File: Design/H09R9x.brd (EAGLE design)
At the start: 34.6 x 30 mm, 24 parts, among them P1 HEXABIT_17.32, U1 STM32F091CBU6, U2 TSD305-1C55, X1 XTALL_CSTCE8M00G52

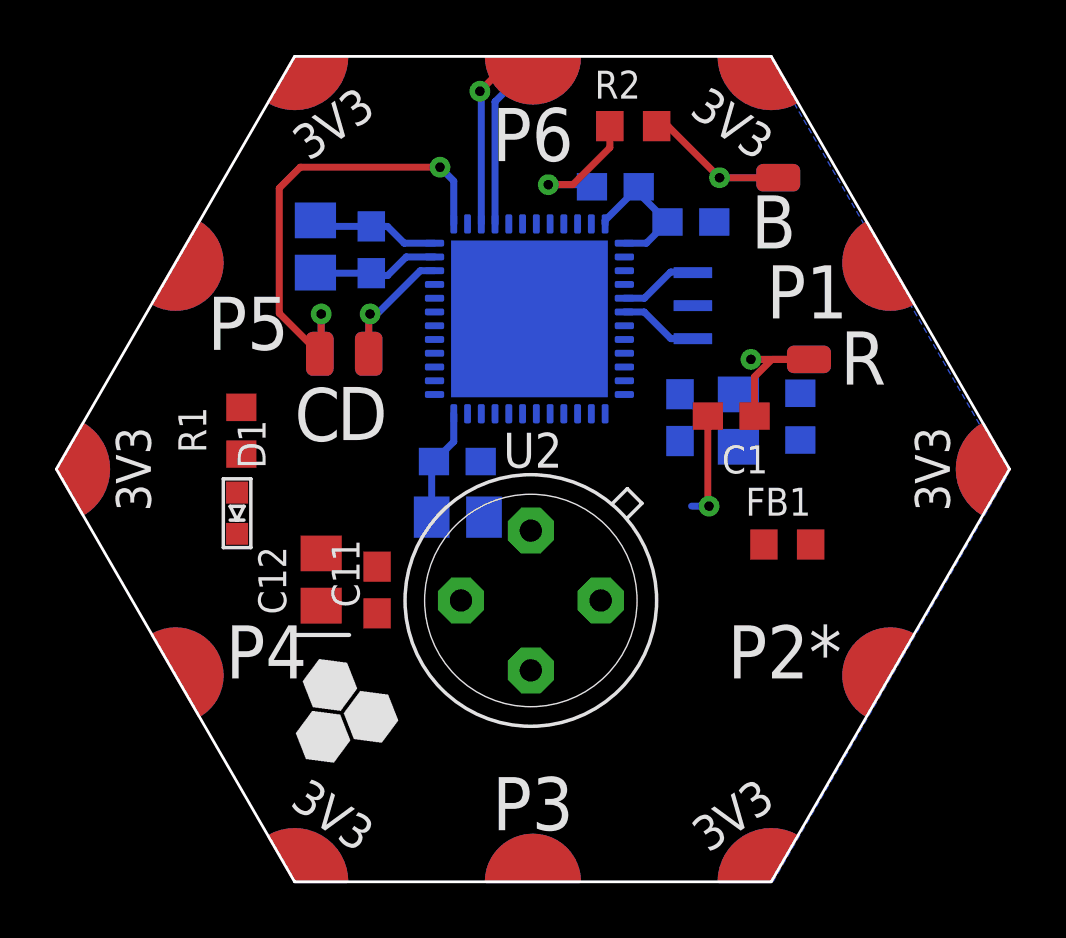
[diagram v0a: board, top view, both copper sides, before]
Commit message: brd edit
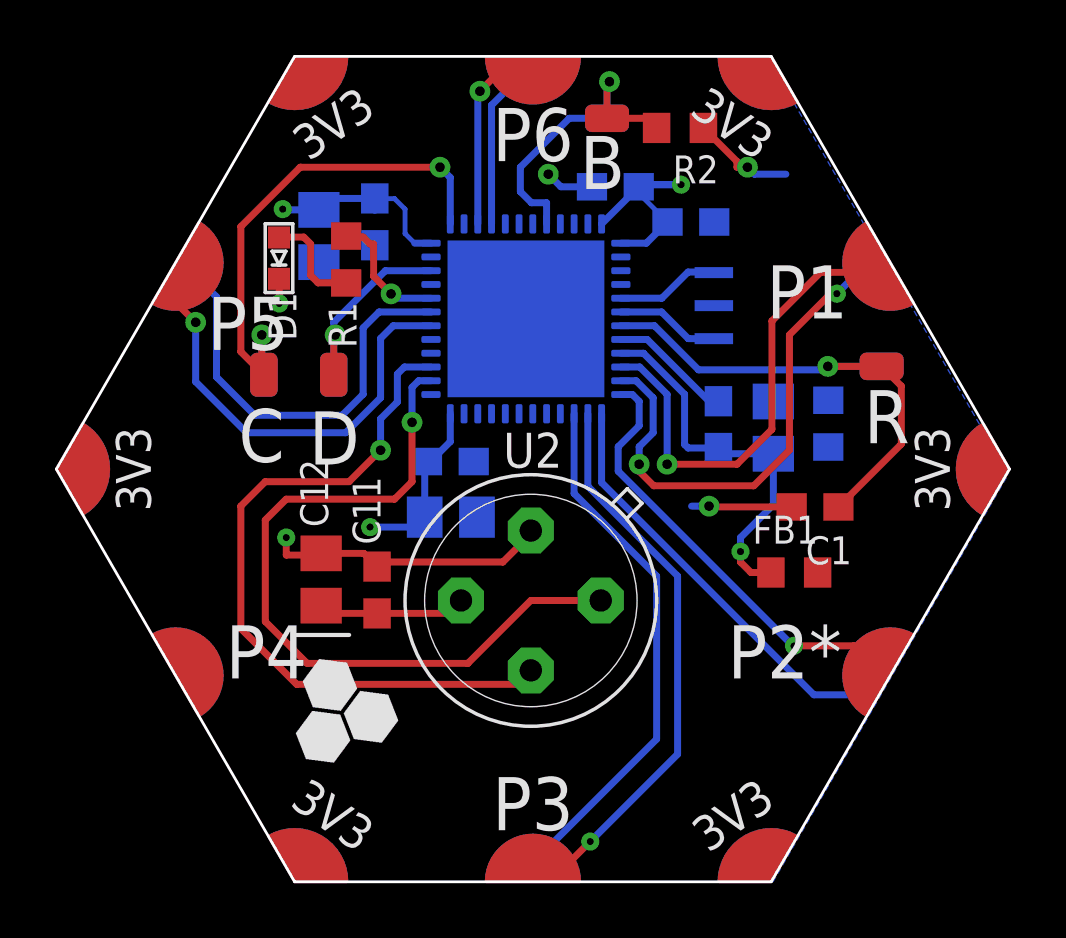
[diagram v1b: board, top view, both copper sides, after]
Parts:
- moved D1 9.40 mm to (25.4, 42.3)
- moved R1 7.30 mm to (27.8, 42.2)
- moved B 6.59 mm to (37.3, 47.4)
- moved C1 4.49 mm to (44.9, 33.2)
- moved R 2.65 mm to (47.3, 38.4), turned to 180 degrees
- moved C 2.17 mm to (24.8, 38.0)
- moved R2 1.70 mm to (40.0, 47.0), turned to 180 degrees
- moved D 1.48 mm to (27.4, 38.0)
- moved C5 1.42 mm to (41.4, 36.2)
- moved C2 1.30 mm to (43.4, 36.1)
- moved FB1 1.05 mm to (44.1, 30.9)
- moved R3 1.05 mm to (45.4, 36.3)
- moved C7 1.02 mm to (28.9, 43.6)
- moved X1 0.76 mm to (41.2, 40.6)
- moved C4 0.40 mm to (26.8, 43.1)
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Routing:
- net I2C2_SCL: track 0.00 -> 27.6 mm, vias 0 -> 1
- net I2C2_SDA: track 0.00 -> 26.3 mm, vias 0 -> 1
- net USART6_TX: track 0.00 -> 20.6 mm, vias 0 -> 1
- net USART6_RX: track 0.00 -> 19.4 mm
- net USART4_RX: track 0.00 -> 18.9 mm, vias 0 -> 2
- net USART4_TX: track 0.00 -> 17.3 mm, vias 0 -> 1
- net USART1_TX: track 0.00 -> 16.5 mm, vias 0 -> 1
- net USART2_RX: track 0.00 -> 16.4 mm
- net USART2_TX: track 0.00 -> 15.9 mm, vias 0 -> 1
- net USART1_RX: track 0.00 -> 15.5 mm
- net VDDA: track 0.00 -> 13.8 mm, vias 0 -> 1
- net VDD: track 14.2 -> 27.7 mm, vias 0 -> 3
- net R1: track 7.88 -> 18.5 mm
- net GND: track 13.8 -> 21.0 mm, vias 2 -> 5
- net N$3: track 0.00 -> 4.71 mm, vias 0 -> 1
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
